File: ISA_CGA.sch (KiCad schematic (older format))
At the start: 21 parts, among them U1 74S112, U11 74LS74, U12 74LS393, U13 74LS08, U14 74LS32, U15 74LS00, U16 74LS04, U26 74LS04, U28 74LS10, U29 74S04, U3 74S86, U30 74LS32, U31 74S08, U41 74LS08, U42 74LS86, U48 74LS51, U49 74LS02, U6 74LS04, U62 74LS125, U65 74LS02, U68 74LS86

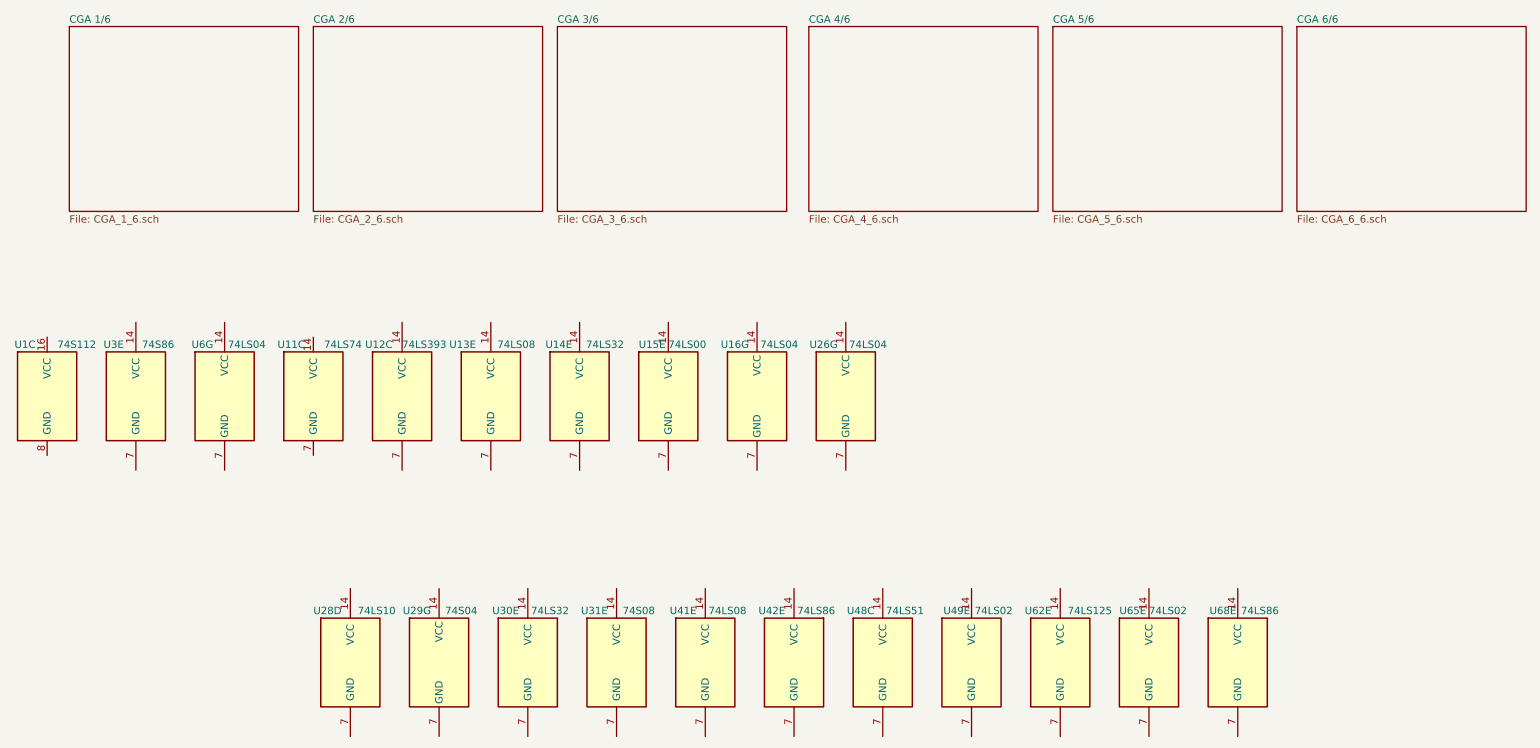
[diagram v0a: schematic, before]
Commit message: More sheet 4
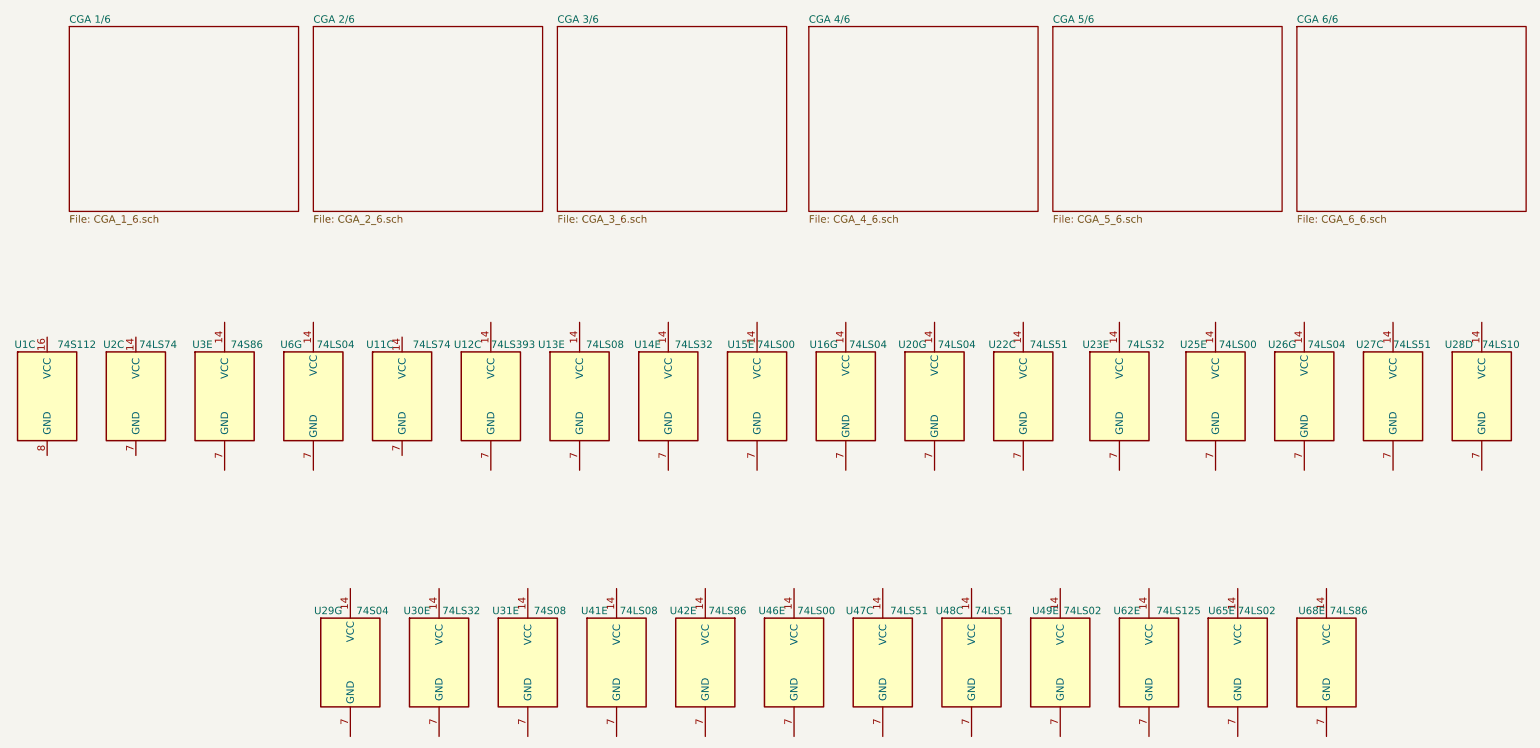
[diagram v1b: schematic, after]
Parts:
- added U2: 74LS74, Package_DIP:DIP-14_W7.62mm_LongPads, symbol 74xx:74LS74
- added U20: 74LS04, Package_DIP:DIP-14_W7.62mm_LongPads, symbol 74xx:74LS04
- added U22, U27, U47: 74LS51, Package_DIP:DIP-14_W7.62mm_LongPads, symbol 74xx:74LS51
- added U23: 74LS32, Package_DIP:DIP-14_W7.62mm_LongPads, symbol 74xx:74LS32
- added U25, U46: 74LS00, Package_DIP:DIP-14_W7.62mm_LongPads, symbol 74xx:74LS00
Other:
- moved on the sheet: U11C, U12C, U13E, U14E, U15E, U16G, U26G, U28D, U30E, U31E, U3E, U41E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
